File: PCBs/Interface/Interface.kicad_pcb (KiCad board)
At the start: 2 copper layers, 43 parts, among them J1 MCU, J2 VLED, SW11 SW_Push, SW13 SW_Push, SW14 SW_Push, SW15 SW_Push, SW16 SW_Push, SW21 SW_Push, SW22 SW_Push, SW23 SW_Push, SW24 SW_Push, SW25 SW_Push, SW26 SW_Push, SW31 SW_Push, SW32 SW_Push, SW35 SW_Push, SW36 SW_Push, SW41 SW_Push, SW42 SW_Push, SW43 SW_Push, SW44 SW_Push, SW45 SW_Push, SW51 SW_Push, SW52 SW_Push, SW53 SW_Push, SW54 SW_Push, SW55 SW_Push, SW56 SW_Push, SW61 SW_Push, SW62 SW_Push, SW63 SW_Push, SW64 SW_Push, SW66 SW_Push

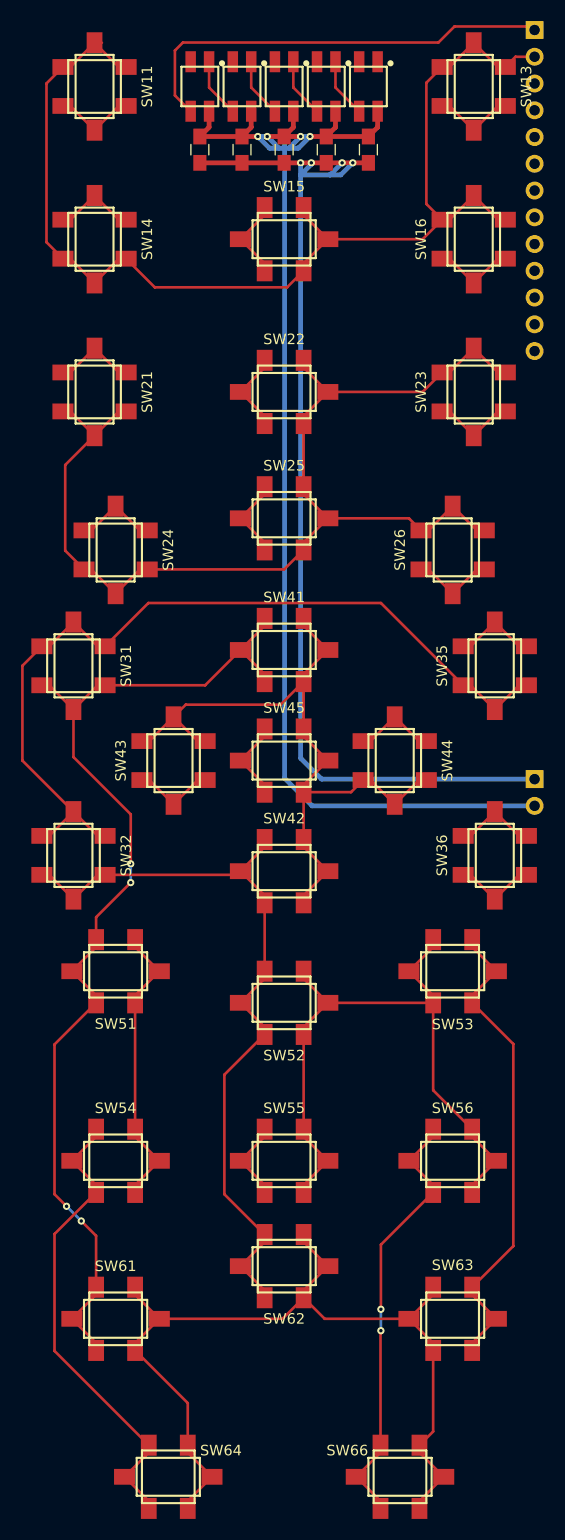
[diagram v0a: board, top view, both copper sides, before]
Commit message: Hopefullly final design before manufacture
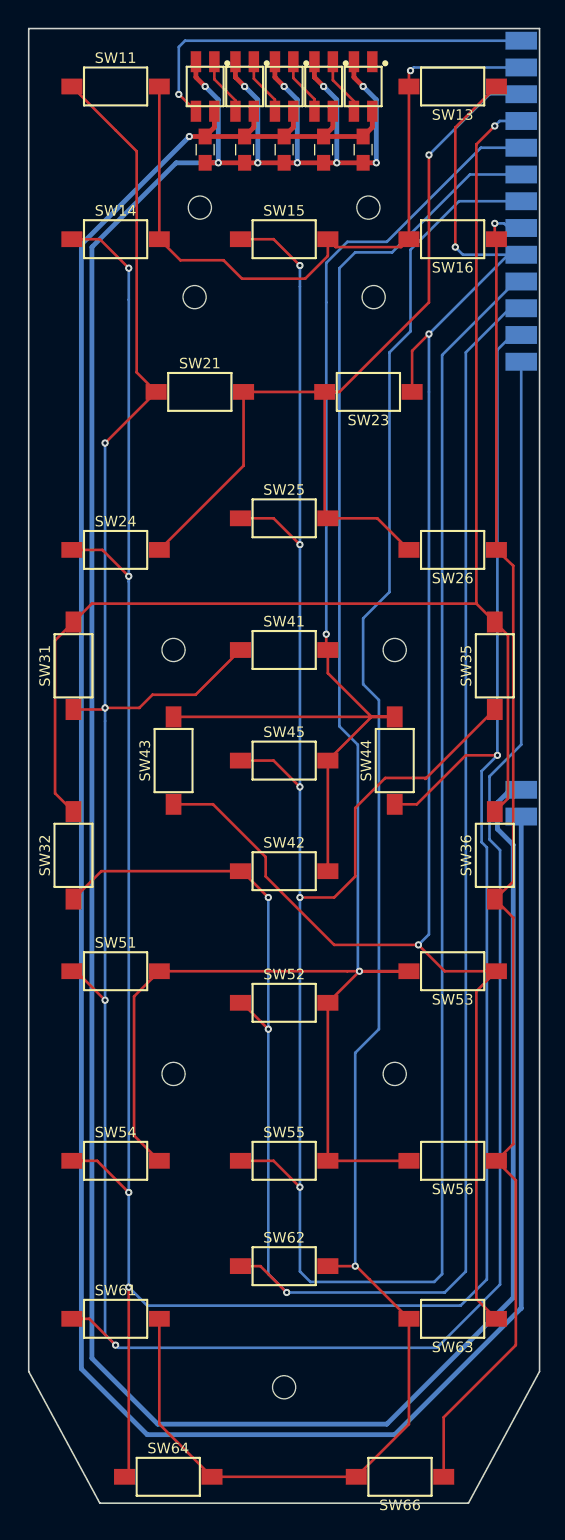
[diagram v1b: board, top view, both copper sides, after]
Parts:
- removed SW22: SW_Push, my-switches:SMD_MultiSwitch
- added REF**: MountingHole_2.2mm_M2, Mounting_Holes:MountingHole_2.2mm_M2, F.Cu at (91.5, 70.0)
- added REF**: MountingHole_2.2mm_M2, Mounting_Holes:MountingHole_2.2mm_M2, F.Cu at (108.5, 70.0)
- added REF**: MountingHole_2.2mm_M2, Mounting_Holes:MountingHole_2.2mm_M2, F.Cu at (108.0, 61.5)
- added REF**: MountingHole_2.2mm_M2, Mounting_Holes:MountingHole_2.2mm_M2, F.Cu at (92.0, 61.5)
- added REF**: MountingHole_2.2mm_M2, Mounting_Holes:MountingHole_2.2mm_M2, F.Cu at (100.0, 173.5)
- added REF**: MountingHole_2.2mm_M2, Mounting_Holes:MountingHole_2.2mm_M2, F.Cu at (89.5, 143.8)
- added REF**: MountingHole_2.2mm_M2, Mounting_Holes:MountingHole_2.2mm_M2, F.Cu at (110.5, 143.8)
- added REF**: MountingHole_2.2mm_M2, Mounting_Holes:MountingHole_2.2mm_M2, F.Cu at (110.5, 103.5)
- added REF**: MountingHole_2.2mm_M2, Mounting_Holes:MountingHole_2.2mm_M2, F.Cu at (89.5, 103.5)
- J1: footprint Pin_Headers:Pin_Header_Angled_1x13_Pitch2.54mm -> my-smd:SMD_Right_Socket_Strip_Angled_1x13_Pitch2.54mm
- J2: footprint Pin_Headers:Pin_Header_Angled_1x02_Pitch2.54mm -> my-smd:SMD_Right_Socket_Strip_Angled_1x02_Pitch2.54mm
- SW11, SW13, SW14, SW15, SW16, SW21, SW23, SW24, SW25, SW26, SW31, SW32, SW35, SW36, SW41, SW42, SW43, SW44, SW45, SW51, SW52, SW53, SW54, SW55, SW56, SW61, SW62, SW63, SW64, SW66: footprint my-switches:SMD_MultiSwitch -> my-switches:SMD_Tactile_Switch
- moved SW21 10.0 mm to (92.0, 79.0), turned to 0 degrees
- moved SW23 10.0 mm to (108.0, 79.0), turned to 180 degrees
- moved SW11 2.00 mm to (84.0, 50.0), turned to 0 degrees
- moved SW13 2.00 mm to (116.0, 50.0), turned to 180 degrees
- moved SW14 2.00 mm to (84.0, 64.5), turned to 0 degrees
- moved SW16 2.00 mm to (116.0, 64.5), turned to 180 degrees
- moved J1 1.63 mm to (122.5, 45.7)
- moved J2 1.63 mm to (122.5, 116.8)
- moved C1 0.50 mm to (92.5, 56.0)
- moved C5 0.50 mm to (107.5, 56.0)
- moved D1 0.50 mm to (92.5, 50.0)
- moved D5 0.50 mm to (107.5, 50.0)
- moved C2 0.25 mm to (96.2, 56.0)
- moved C4 0.25 mm to (103.8, 56.0)
- moved D2 0.25 mm to (96.2, 50.0)
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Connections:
- J1 pad 10: /COL3 -> /COL5
- J1 pad 11: /COL4 -> /COL2
- J1 pad 12: /COL5 -> /COL4
- J1 pad 13: /COL6 -> /COL1
- J1 pad 8: /COL1 -> /COL6
- J1 pad 9: /COL2 -> /COL3
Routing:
- net /COL5: track 39.5 -> 264.0 mm, vias 0 -> 5
- net /COL4: track 68.9 -> 274.2 mm, vias 0 -> 5
- net /GND: track 104.2 -> 287.4 mm, vias 4 -> 10
- net /COL1: track 117.4 -> 281.8 mm
- net /VLED: track 127.7 -> 247.6 mm, vias 4 -> 1
- net /COL3: track 69.8 -> 172.9 mm, vias 0 -> 3
- net /COL2: track 81.2 -> 180.5 mm, vias 0 -> 3
- net /ROW6: track 85.5 -> 169.9 mm, vias 0 -> 1
- net /ROW5: track 92.0 -> 163.8 mm, vias 0 -> 1
- net /COL6: track 65.6 -> 128.2 mm, vias 2 -> 1
- net /ROW3: track 89.0 -> 128.7 mm, vias 0 -> 1
- net /ROW1: track 108.9 -> 69.6 mm, vias 0 -> 1
- net /ROW4: track 68.4 -> 107.5 mm, vias 0 -> 1
- net /ROW2: track 104.6 -> 86.6 mm, vias 0 -> 1
- net /DIN1: track 41.6 -> 39.5 mm, vias 0 -> 1
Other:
- board outline added: 48.5 x 140 mm
